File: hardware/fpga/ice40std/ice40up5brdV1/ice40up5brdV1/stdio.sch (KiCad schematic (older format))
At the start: 17 parts, among them J1 Conn_01x20_Male, J2 Conn_01x20_Female, SW1 SW_Push, SW2 SW_Push, SW3 SW_Push

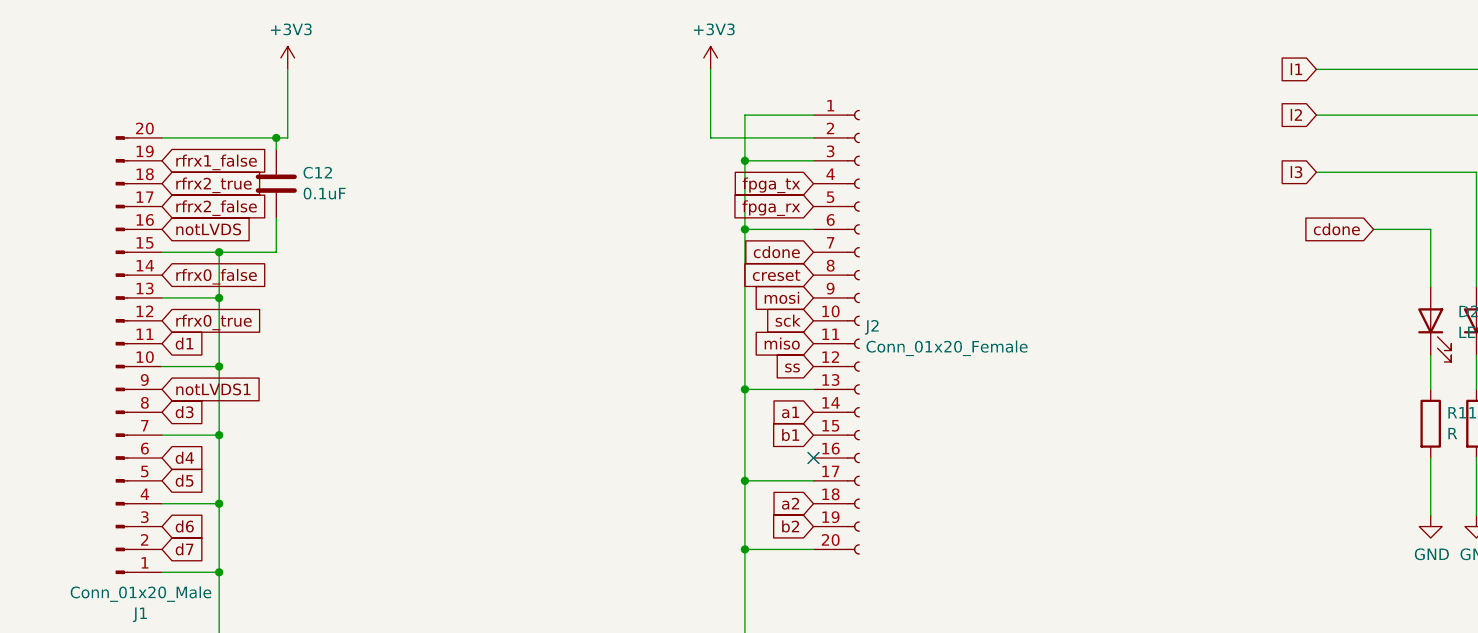
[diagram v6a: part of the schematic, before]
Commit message: ice40qfn restarted: simplest design ready?
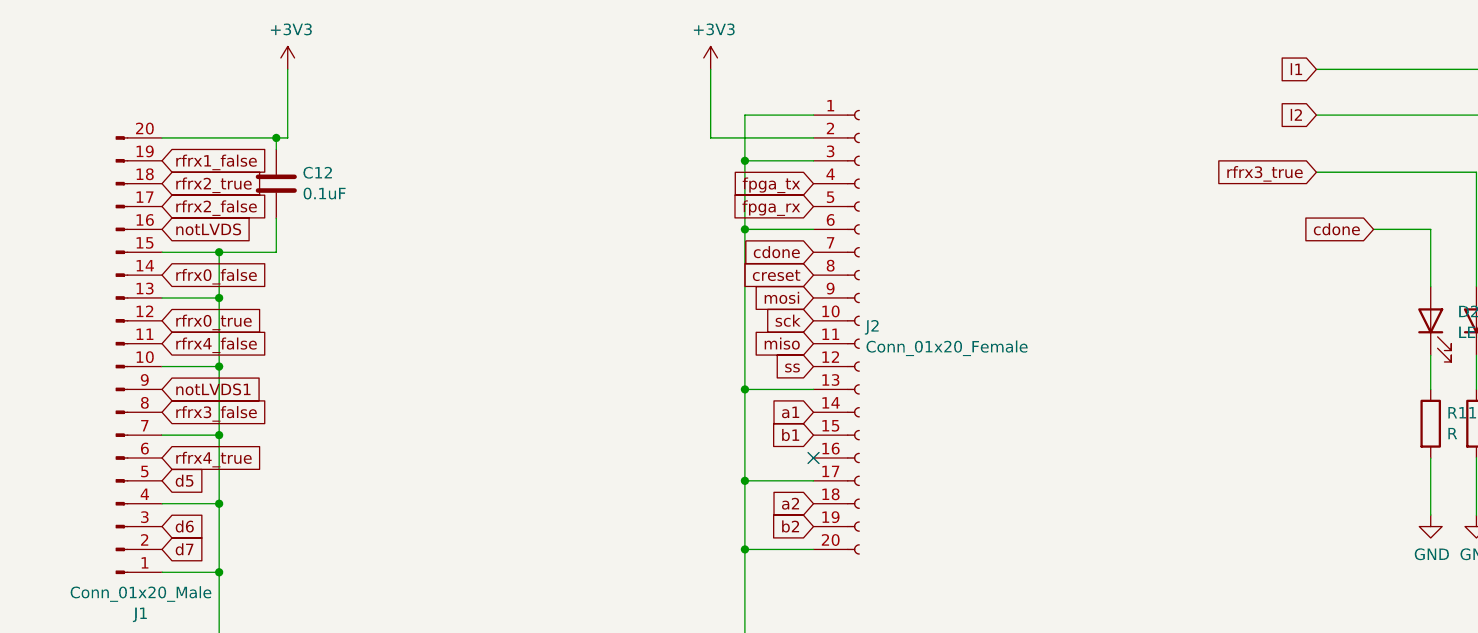
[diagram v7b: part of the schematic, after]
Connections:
- net d1 renamed rfrx4_false
- net d3 renamed rfrx3_false
- net d4 renamed rfrx4_true
- net l3 renamed rfrx3_true
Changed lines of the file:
@@
 l2
 Text GLabel 7700 2300 0    50   Input ~ 0
-l3
+rfrx3_true
 Wire Wire Line
 	7700 2300 8400 2300
@@
 rfrx0_true
 Text GLabel 2650 3050 2    50   Input ~ 0
-d1
+rfrx4_false
 Text GLabel 2650 3250 2    50   Input ~ 0
 notLVDS1
 Text GLabel 2650 3350 2    50   Input ~ 0
-d3
+rfrx3_false
 Text GLabel 2650 3550 2    50   Input ~ 0
-d4
+rfrx4_true
 Text GLabel 2650 3650 2    50   Input ~ 0
 d5

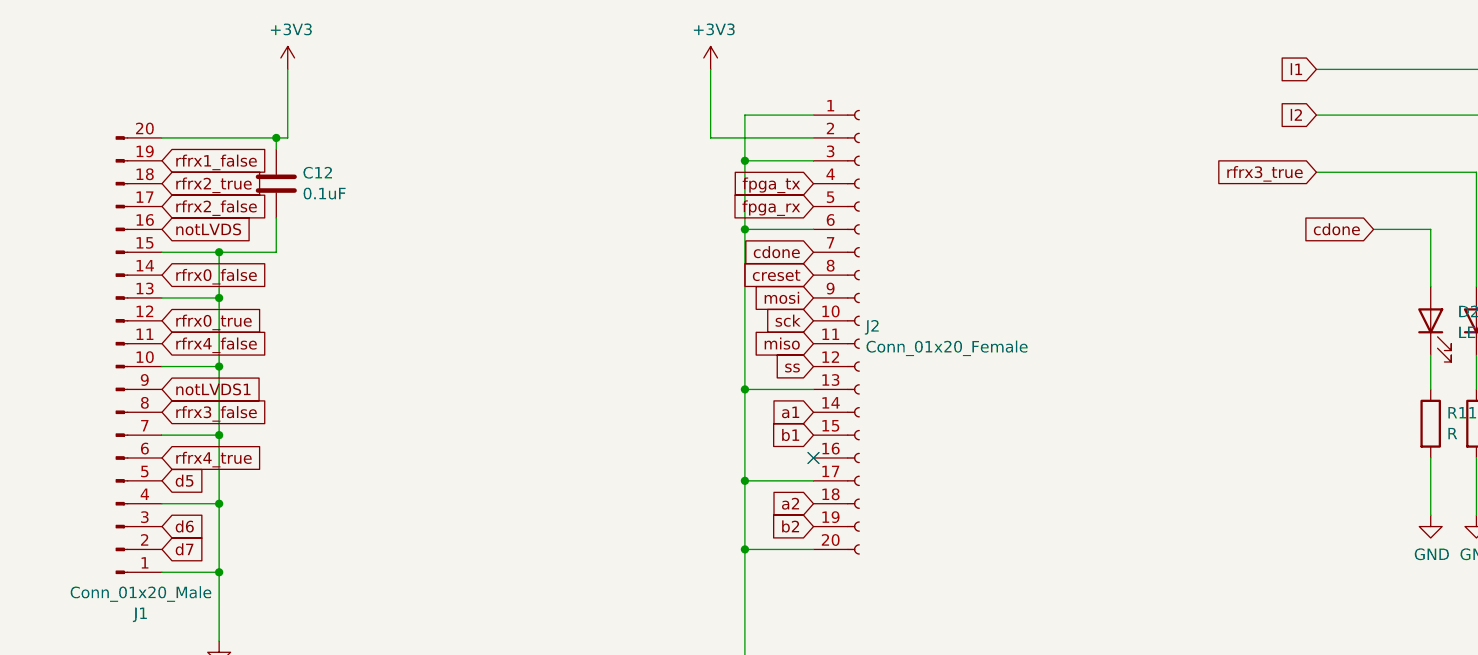
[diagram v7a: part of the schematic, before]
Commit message: ice40qfn restarted: simplest design ready?
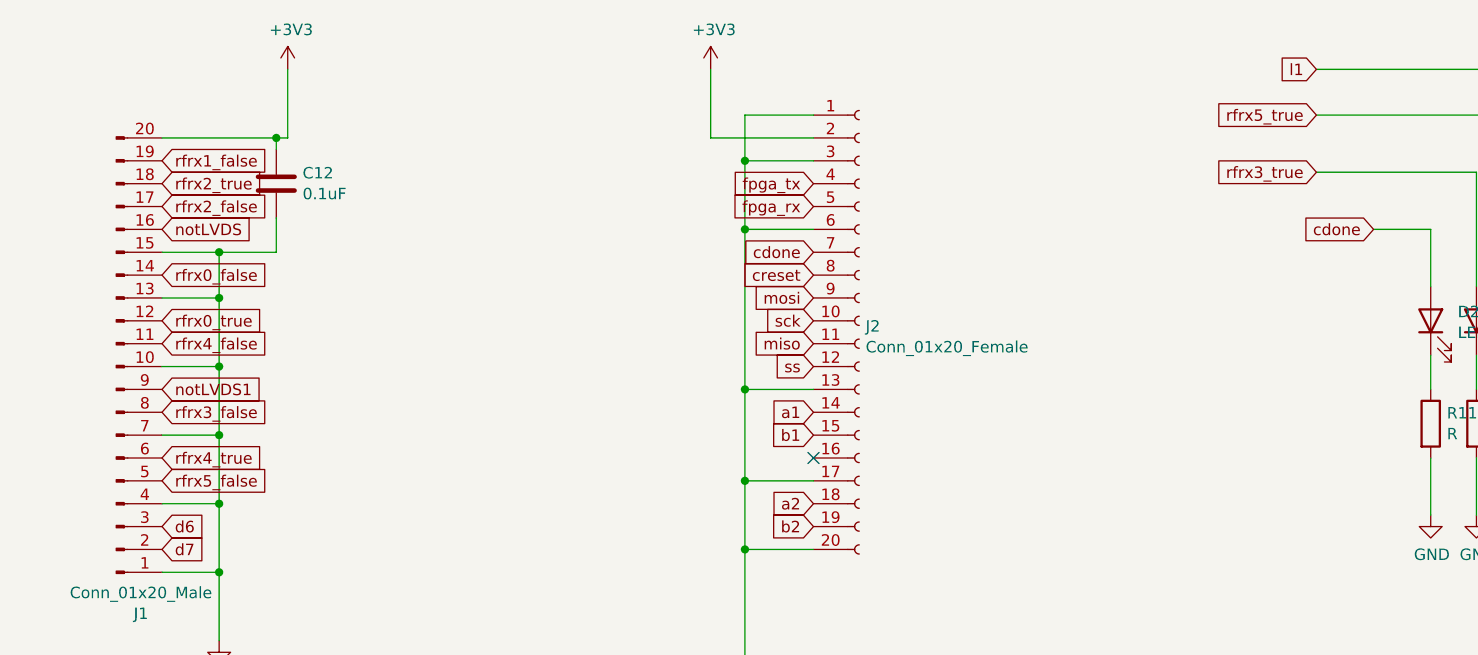
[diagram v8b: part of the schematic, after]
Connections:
- net d5 renamed rfrx5_false
- net l2 renamed rfrx5_true
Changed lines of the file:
@@
 l1
 Text GLabel 7700 2050 0    50   Input ~ 0
-l2
+rfrx5_true
 Text GLabel 7700 2300 0    50   Input ~ 0
 rfrx3_true
@@
 rfrx4_true
 Text GLabel 2650 3650 2    50   Input ~ 0
-d5
+rfrx5_false
 Text GLabel 2650 3850 2    50   Input ~ 0
 d6
